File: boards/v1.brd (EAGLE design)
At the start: 24.2 x 49.6 mm, 48 parts, among them IC2 LT1761, IC4 LT1376-ADJ, Q1 12Mhz, T1 Si2301DS, X1 USB-MICROB

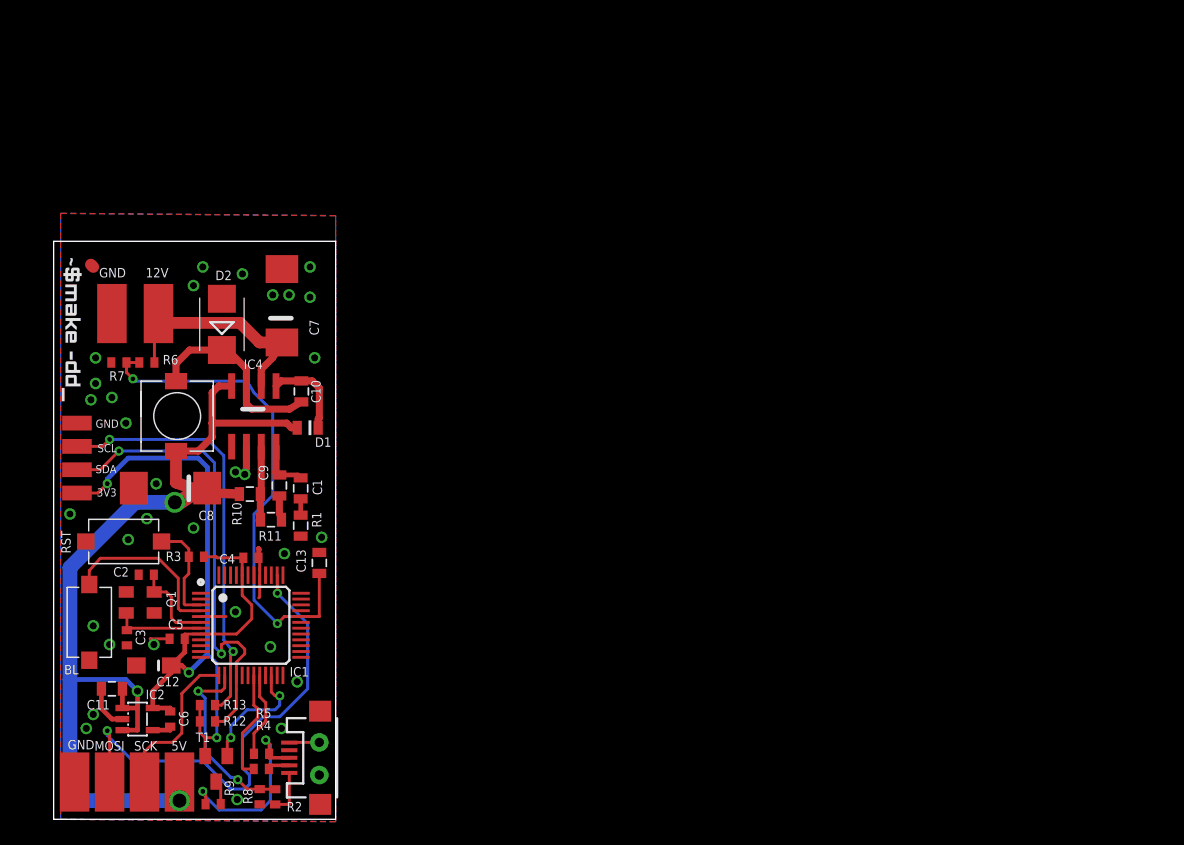
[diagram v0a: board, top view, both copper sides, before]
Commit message: put all the downloaded files into directories
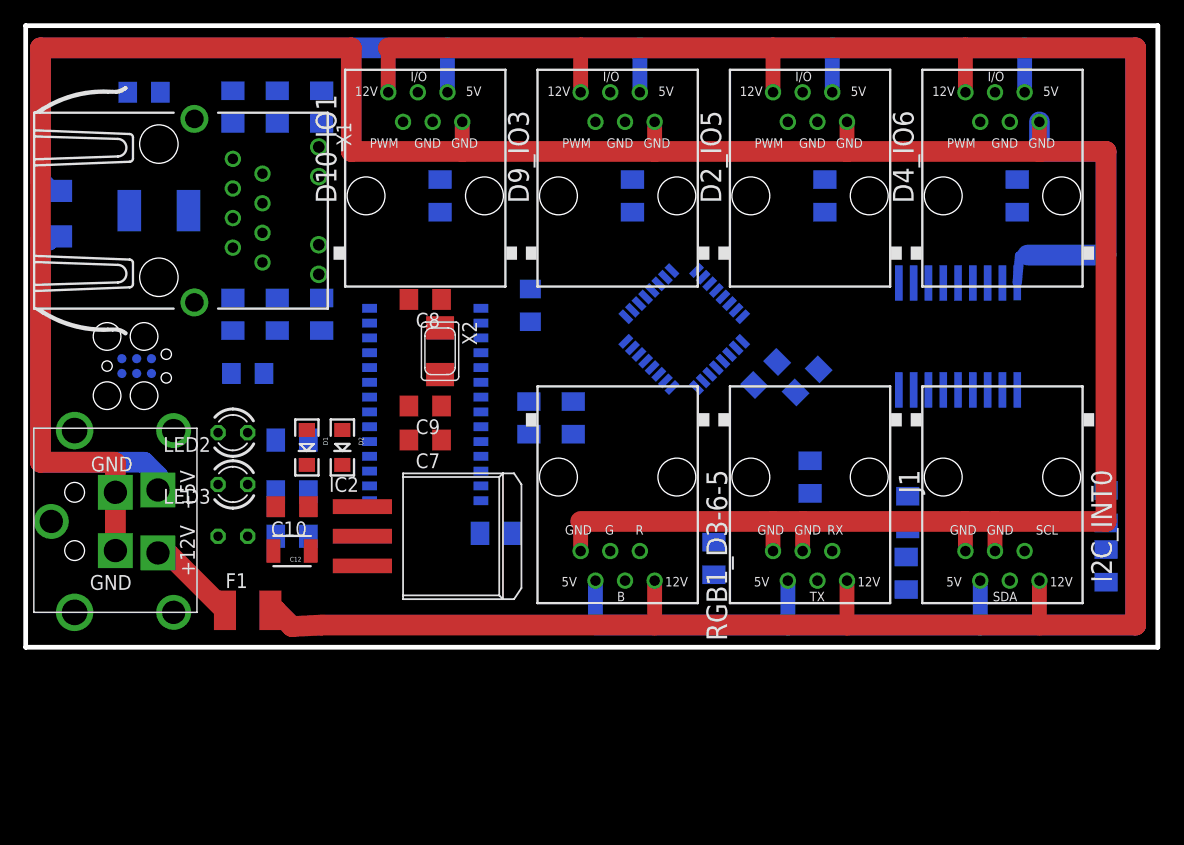
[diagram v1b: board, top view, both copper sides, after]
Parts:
- removed 12V, 5V, GND, GND1, MOSI, SCK: (no value), wirepad:SMD2,54-5,08
- removed 3V3, GN, SCL, SDA: (no value), wirepad:SMD1,27-2,54
- removed BL, RST: SWITCH_MCTAEF, seb:SWITCH_MCTAEF
- removed C11, C13: 1µF, SparkFun-Capacitors:0805
- removed C3: 22pF, rcl:C0402
- removed IC4: LT1376-ADJ, v-reg:SO-08
- removed L2: 20µH/xxx mA, seb:PIS2408
- removed Q1: 12Mhz, seb:MT
- removed T1: Si2301DS, SparkFun:SOT23
- removed U$1: MAKE-DD_LOGO'PROMPT', seb:MAKE-DD_LOGO_PROMPT
- added CON2: (no value), lpatiny:TC2030-MCP
- added D10_IO1: IO1, lpatiny:RJ12-STRAIGHT
- added D2_IO5: IO5, lpatiny:RJ12-STRAIGHT
- added D4_IO6: IO6, lpatiny:RJ12-STRAIGHT
- added D9_IO3: IO3, lpatiny:RJ12-STRAIGHT
- added F1, F2: POLYSWITCHSMD1812, lpatiny:C1812
- added I2C_INT0: I2C, lpatiny:RJ12-STRAIGHT-I2C
- added IC3: ULN2803A, lpatiny:SO18W
- added J1: RJ12STRAIGHT-RS232-SERVER, lpatiny:RJ12-STRAIGHT-RS232
- added L1: 10uH, SparkFun:INDUCTOR-1206
- added LED2, LED3, LED5: (no value), lpatiny:LED3MM
- added R0, R18, R1B, RL2, RL3: 1K, resistor:M1206
- added R14, R15: 50, resistor:M1206
- added R16: 2k, resistor:M1206
- added R19: 100k, resistor:M1206
- added RGB1_D3-6-5: RGB1, lpatiny:RJ12-STRAIGHT-RGB
- added U$2: KPJX-4S-S, lpatiny:KPJX-4S-S
- added U1: (no value), lpatiny:SO28W
- added X2: (no value), adafruit:NX5032
- C1: value 3,3nF -> 0.1uF; device SparkFun:0805 -> resistor:C1206
- C10: value 100nF -> 470nF; device SparkFun:0805 -> rcl:C1206
- C12: value (none) -> 33uF; device rcl:SMC_A -> SparkFun:1210
- C2: value 22pF -> 0.1uF; device rcl:C0402 -> resistor:C1206
- C4, C5: value 100nF -> 10nF; device rcl:C0402 -> resistor:C1206
- C6: value 10nF -> 10uF; device rcl:C0402 -> resistor:C1206
- C7: value 10µF/35V -> 100nF; device resistor:SMC_D -> resistor:C1206
- C8: value 100µF/6V -> 18pF; device resistor:SMC_D -> resistor:C1206
- C9: value 470pF -> 18pF; device SparkFun:0805 -> resistor:C1206
- D1: value 4148 -> 1N581D1206; device seb:DIODE_0805 -> lpatiny:LED-1206
- D2: value MBRS140 -> 1N581D1206; device diode:SMB -> lpatiny:LED-1206
- IC1: value (none) -> MEGA8-AI; device microbuilder:LQFP48 -> atmel:TQFP32-08
- IC2: value LT1761 -> LM3940IS-3.3F; device seb:SOT23-5L -> lpatiny:DD-3
- R1: value 3,3k -> 10k; device SparkFun:0805 -> resistor:M1206
- R10: value 1k82 -> 470; device SparkFun:0805 -> resistor:M1206
- R11: value 5k -> 470; device SparkFun:0805 -> resistor:M1206
- R12, R13: value 15k -> 50; device rcl:R0402 -> resistor:M1206
- R2, R3: value 15k -> 1K; device rcl:R0402 -> resistor:M1206
- R4, R5: value 33R -> 1K; device rcl:R0402 -> resistor:M1206
- R6: value 680k -> 1K; device rcl:R0402 -> resistor:M1206
- R7: value 220k -> 10K; device rcl:R0402 -> resistor:M1206
- R8: value 15k -> 10K; device rcl:R0402 -> resistor:M1206
- R9: value 1k5 -> 1K; device rcl:R0402 -> resistor:M1206
- X1: value USB-MICROB -> hy911103a; device SparkFun-Connectors:USB-MICROB -> con-pulse:J1
- moved R7 85.6 mm to (92.7, 11.4), flipped to the bottom, turned to 90 degrees
- moved R6 84.1 mm to (92.7, 6.35), flipped to the bottom, turned to 90 degrees
- moved R2 59.5 mm to (75.7, 10.9), flipped to the bottom, turned to 270 degrees
- moved C2 59.1 mm to (67.1, 22.2), flipped to the bottom, turned to 315 degrees
- moved R8 58.7 mm to (75.6, 5.71), flipped to the bottom, turned to 270 degrees
- moved R4 58.6 mm to (52.1, 38.1), flipped to the bottom, turned to 270 degrees
- moved R9 55.7 mm to (35.6, 38.1), flipped to the bottom, turned to 270 degrees
- moved R12 52.8 mm to (17.8, 45.7), flipped to the bottom, turned to 90 degrees
- moved R5 52.7 mm to (67.3, 14.0), flipped to the bottom, turned to 90 degrees
- moved R13 51.7 mm to (21.6, 45.7), flipped to the bottom, turned to 90 degrees
- moved X1 47.5 mm to (17.8, 36.8), turned to 270 degrees
- moved C6 47.1 mm to (43.3, 28.7), flipped to the bottom, turned to 270 degrees
- moved IC1 45.0 mm to (56.5, 26.7), flipped to the bottom, turned to 225 degrees
- moved R3 44.4 mm to (59.1, 6.99), flipped to the bottom, turned to 90 degrees
- moved C1 41.1 mm to (63.5, 22.9), flipped to the bottom, turned to 315 degrees
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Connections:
- removed net +5V_USB: R2.1, X1.VBUS
- removed net 01: BL.2, IC1.4
- removed net 06: IC1.22, T1.1
- removed net ADC: C13.1, IC1.32, R6.2, R7.2
- removed net N$20: R9.2, T1.3
- removed net N$24: IC1.20, R5.1
- removed net N$3: C3.2, IC1.7, Q1.1
- removed net N$56: C1.1, C9.1, IC4.8
- removed net N$57: C10.2, D2.C, IC4.3, L2.P$1
- removed net N$58: C10.1, D1.1, IC4.1
- removed net N$7: IC1.13, SCK.1
- removed net RST: IC1.3, R3.1, RST.2
- removed net VBUS: IC1.14, R2.2, R8.2
- new net 3.3V: C7.1, U1.15, U1.19, U1.20, U1.28
- new net 5V: R7.2, R8.2
- new net A0: IC1.23, R0.2
- new net A1: IC1.24, R1B.2
- new net A2: IC1.25, R4.2
- new net A3: IC1.26, R9.2
- new net A6: IC1.19
- new net A7: IC1.22
- new net COM: IC3.10
- new net D10: IC1.14, R19.1, U1.9
- new net D2: IC1.32, IC3.5
- new net D2B: D9_IO3.I/O, R4.1
- new net D2B1: D10_IO1.I/O, R9.1
- new net D2B4: I2C_INT0.SDA, R2.1
- new net D2B5: J1.TX, R3.1
- new net D2B6: D2_IO5.I/O, R0.1
- new net D2B7: D4_IO6.I/O, R1B.1
- new net D3: IC1.1, IC3.1
- new net D4: IC1.2, IC3.6
- new net D5: IC1.9, IC3.3
- new net D6: IC1.10, IC3.2
- new net D7: IC1.11, IC3.8
- new net D8: IC1.12, IC3.4
- new net D9: IC1.13, IC3.7
- new net ISP+5V: CON2.5V, D1.A
- new net MISO: CON2.MISO, IC1.16, U1.6
- new net MOSI: CON2.MOSI, IC1.15, U1.7
- new net N$12: R11.1, X1.12
- new net N$13: R15.1, U1.17, X1.1
- new net N$15: R13.1, U1.13, X1.7
- new net N$16: R12.1, U1.12, X1.8
- new net N$17: C4.2, L1.P$2, R12.2, R13.2, X1.3
- new net N$18: C5.2, R14.2, R15.2
- new net N$19: C10.1, D1.C, D2.C, IC2.1
- new net N$22: D9_IO3.PWM, IC3.12
- new net N$26: C6.1, U1.1
- new net N$27: R16.2, U1.14
- new net N$28: C9.1, U1.23, X2.P$1
- new net N$29: C8.1, U1.24, X2.P$2
- new net N$5: LED5.A, R18.1
- new net N$50: IC3.17, RGB1_D3-6-5.B
- new net N$51: D10_IO1.PWM, IC3.11
- new net N$60: D2_IO5.PWM, IC3.14
- new net N$68: IC3.18, RGB1_D3-6-5.R
- new net N$70: J1.RX, R5.1
- new net N$71: I2C_INT0.SCL, R6.1
- new net N$75: LED3.A, RL3.1
- new net N$76: LED2.A, RL2.1
- new net N$9: R10.2, U1.27
- new net RESET: CON2.RESET, IC1.29, R1.1, U1.10
- new net RX: IC1.30, R5.2
- new net SCK: CON2.SCK, IC1.17, U1.8
- new net TX: IC1.31, R3.2
- net +12V: now also D10_IO1.+12V, D2_IO5.+12V, D4_IO6.+12V, D9_IO3.+12V, F1.2, I2C_INT0.+12V, J1.+12V, RGB1_D3-6-5.+12V, RL3.2; no longer 12V.1, C7.+, IC4.2, R6.1
- net +3V3: now also C1.1, C12.1, C2.1, IC1.18, IC1.4, IC1.6, IC2.3, L1.P$1, R1.2, R18.2, R19.2, U1.25; no longer 3V3.1, C12.+, C4.2, C5.2, C6.2, IC1.44, IC1.8, IC2.5, R12.1, R13.1, R3.2, T1.2
- net +5V: now also D10_IO1.+5V, D2.A, D2_IO5.+5V, D4_IO6.+5V, D9_IO3.+5V, F2.2, I2C_INT0.+5V, J1.+5V, RGB1_D3-6-5.+5V, RL2.2; no longer 5V.1, C11.1, C8.+, D1.2, IC2.1, IC2.3, IC4.4, L2.P$2, R10.2
- net GND: now also C10.2, C12.2, C2.2, C6.2, C7.2, C8.2, CON2.GND, D10_IO1.GND1, D10_IO1.GND2, D2_IO5.GND1, D2_IO5.GND2, D4_IO6.GND1, D4_IO6.GND2, D9_IO3.GND1, D9_IO3.GND2, I2C_INT0.GND1, I2C_INT0.GND2, IC1.21, IC1.3, IC3.9, J1.GND1, J1.GND2, LED2.K, LED3.K, LED5.K, R16.1, RGB1_D3-6-5.GND1, U$2.GND1, U$2.GND2, U1.11, U1.18, U1.2, U1.21, U1.22, X1.10, X1.11; no longer BL.1, C11.2, C12.-, C13.2, C2.1, C3.1, C7.-, C8.-, D2.A, GN.1, GND.1, GND1.1, IC1.41, IC4.6, R1.1, R11.1, R7.1, R8.1, RST.1, X1.GND, X1.MT1, X1.MT2
- net N$1: now also IC3.16, RGB1_D3-6-5.G; no longer C1.2, R1.2
- net N$10: now also U1.26; no longer IC4.7, R10.1
- net N$11: now also R10.1, X1.9; no longer R4.2, X1.D-
- net N$14: now also R14.1, U1.16, X1.2; no longer IC1.19, R4.1
- net N$2: now also D4_IO6.PWM, IC3.13; no longer R5.2, R9.1, X1.D+
- net N$4: now also C1.2, IC1.20; no longer C2.2, IC1.6, Q1.3
- net N$6: now also F2.1, U$2.+5V; no longer C6.1, IC2.4
- net N$8: now also F1.1, U$2.+12V; no longer IC1.38, MOSI.1
- net SCL: now also IC1.28, R6.2, R7.1; no longer IC1.15, R13.2, SCL.1
- net SDA: now also IC1.27, R2.2, R8.1; no longer IC1.16, R12.2, SDA.1
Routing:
- net GND: track 20.4 -> 276.4 mm, vias 34 -> 0
- net +12V: track 20.7 -> 215.2 mm
- net +5V: track 83.8 -> 229.3 mm, vias 3 -> 0
- net +3V3: track 70.8 -> 0.00 mm, vias 3 -> 0
- net ADC: track 43.3 -> 0.00 mm, vias 2 -> 0
- net SDA: track 40.3 -> 0.00 mm, vias 2 -> 0
- net SCL: track 36.1 -> 0.00 mm, vias 2 -> 0
- net N$8: track 41.5 -> 7.79 mm, vias 2 -> 0
- net N$6: track 1.80 -> 32.0 mm
- net N$2: track 16.8 -> 0.00 mm, vias 2 -> 0
- net N$57: track 16.8 -> 0.00 mm
- net VBUS: track 16.4 -> 0.00 mm, vias 2 -> 0
- net 01: track 14.6 -> 0.00 mm
- net N$7: track 13.7 -> 0.00 mm
- net 06: track 10.7 -> 0.00 mm, vias 2 -> 0
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- removed copper zone on layer 1, net GND
- removed copper zone on layer 16, net GND
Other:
- board size 24.2 x 49.6 mm -> 97.2 x 53.3 mm
- board text removed: "12Mhz"
- board text removed: "GND"
- board text removed: "Q1"
- board text removed: "lpc1347"
